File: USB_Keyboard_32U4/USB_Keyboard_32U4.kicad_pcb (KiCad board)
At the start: 2 copper layers, 36 x 14.2 mm, 14 parts, among them J1 USB_C_Receptacle_USB2.0_16P, J2 Conn_02x03_Odd_Even, U1 ATmega32U4-A, Y1 16mhz

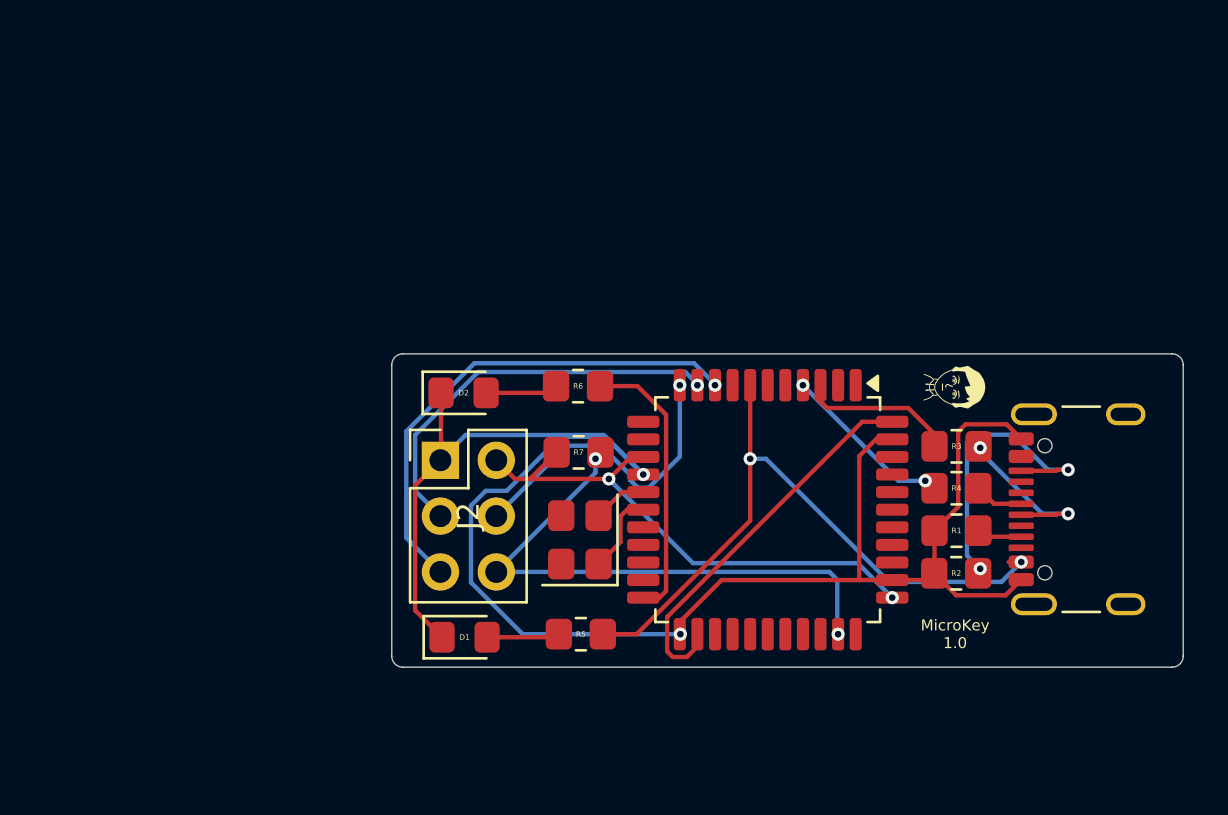
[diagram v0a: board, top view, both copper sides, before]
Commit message: Updated schematic, pcb and bom.
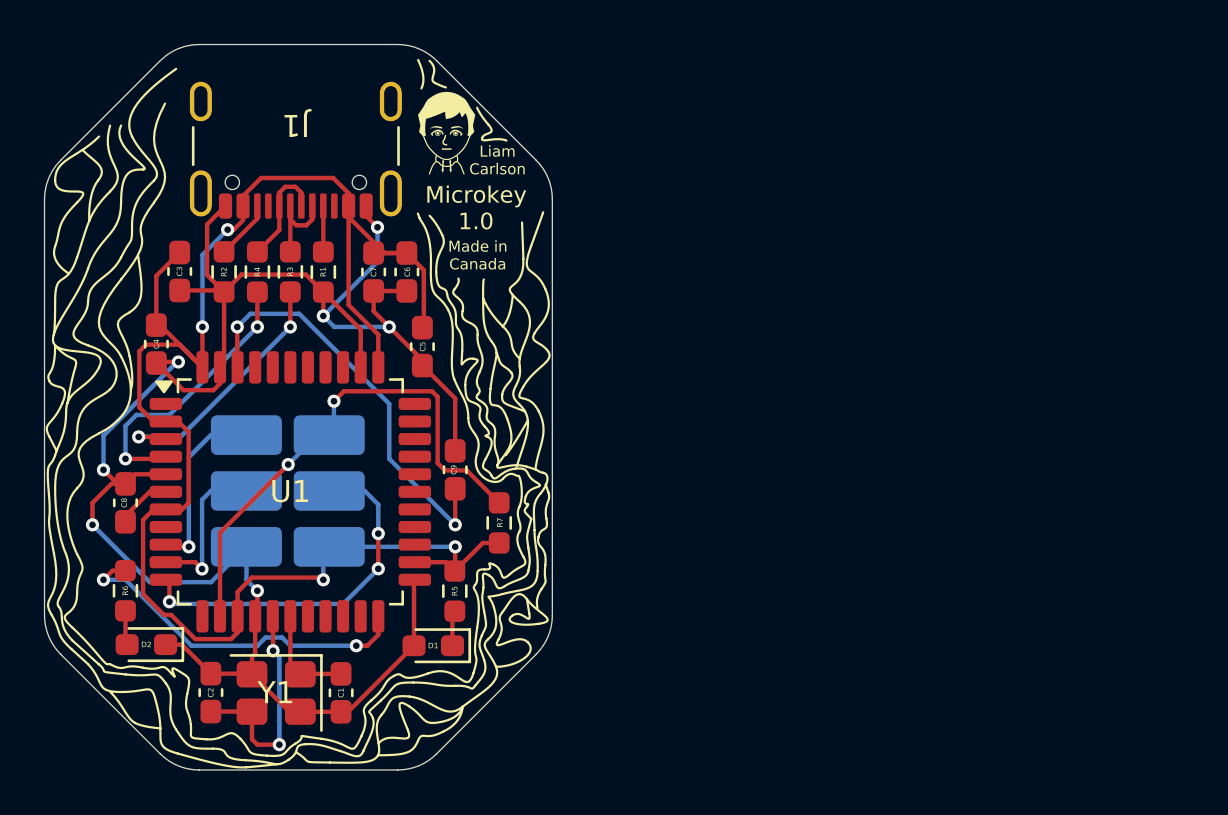
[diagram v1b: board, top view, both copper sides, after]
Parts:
- removed the G*** at (194.5, 132.9)
- added C1: 27pF, Capacitor_SMD:C_0603_1608Metric_Pad1.08x0.95mm_HandSolder, F.Cu at (166.5, 146.8)
- added C2: 27pF, Capacitor_SMD:C_0603_1608Metric_Pad1.08x0.95mm_HandSolder, F.Cu at (160.6, 146.8)
- added C3: 100nF, Capacitor_SMD:C_0603_1608Metric_Pad1.08x0.95mm_HandSolder, F.Cu at (159.2, 127.6)
- added C4: 100nF, Capacitor_SMD:C_0603_1608Metric_Pad1.08x0.95mm_HandSolder, F.Cu at (158.1, 130.9)
- added C5: 100nF, Capacitor_SMD:C_0603_1608Metric_Pad1.08x0.95mm_HandSolder, F.Cu at (170.2, 131.1)
- added C6: 100nF, Capacitor_SMD:C_0603_1608Metric_Pad1.08x0.95mm_HandSolder, F.Cu at (169.5, 127.7)
- added C7: 10uF, Capacitor_SMD:C_0603_1608Metric_Pad1.08x0.95mm_HandSolder, F.Cu at (168.0, 127.7)
- added C8: 1uF, Capacitor_SMD:C_0603_1608Metric_Pad1.08x0.95mm_HandSolder, F.Cu at (156.7, 138.2)
- added C9: 100nF, Capacitor_SMD:C_0603_1608Metric_Pad1.08x0.95mm_HandSolder, F.Cu at (171.7, 136.7)
- added G***: LOGO, Custom Footprints:MIIImage 8.25mm, F.Cu at (171.3, 121.1)
- D1, D2: footprint LED_SMD:LED_0805_2012Metric_Pad1.15x1.40mm_HandSolder -> LED_SMD:LED_0603_1608Metric_Pad1.05x0.95mm_HandSolder
- J2: footprint Connector_PinHeader_2.54mm:PinHeader_2x03_P2.54mm_Vertical -> 2x3 Pads:MicroKey_AVR_ISP_2x3_SMD; moved to B.Cu
- R1, R2, R3, R4, R5, R6: footprint Resistor_SMD:R_0805_2012Metric_Pad1.20x1.40mm_HandSolder -> Resistor_SMD:R_0603_1608Metric_Pad0.98x0.95mm_HandSolder
- R7: value 1k -> 10k; footprint Resistor_SMD:R_0805_2012Metric_Pad1.20x1.40mm_HandSolder -> Resistor_SMD:R_0603_1608Metric_Pad0.98x0.95mm_HandSolder
- Y1: value 16mhz -> 16MHz
- moved J1 40.6 mm to (164.4, 121.0), turned to 180 degrees
- moved R2 36.0 mm to (161.2, 127.7), turned to -90 degrees
- moved R4 32.8 mm to (162.7, 127.7), turned to -90 degrees
- moved R3 31.9 mm to (164.2, 127.7), turned to -90 degrees
- moved R1 31.1 mm to (165.7, 127.7), turned to -90 degrees
- moved R6 22.6 mm to (156.7, 142.2), turned to -90 degrees
- moved U1 21.7 mm to (164.2, 137.7), turned to 0 degrees
- moved D2 18.4 mm to (157.7, 144.6), turned to 180 degrees
- moved Y1 15.5 mm to (163.6, 146.8), turned to 180 degrees
- moved J2 7.08 mm to (164.1, 137.6)
- moved R5 6.06 mm to (171.7, 142.2), turned to -90 degrees
- moved R7 4.83 mm to (173.7, 139.1), turned to 90 degrees
- moved D1 1.48 mm to (170.7, 144.7), turned to 180 degrees
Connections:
- net /unconnected-(U1-PD5-Pad22) renamed Net-(U1-PD5)
- net Net-(J2-Pin_3) renamed PB2
- net Net-(J2-Pin_4) renamed PB3
- net Net-(J2-Pin_5) renamed PB1
- D1 pad 1: /Net-(J1-GND-PadA1) -> Net-(D1-K)
- D1 pad 2: Net-(D1-A) -> GND
- D2 pad 1: /Net-(J1-GND-PadA1) -> GND
- J1 pad A1: /Net-(J1-GND-PadA1) -> GND
- J1 pad A12: /Net-(J1-GND-PadA1) -> GND
- J1 pad A4: Net-(U1-VBUS) -> VCC
- J1 pad A9: Net-(U1-VBUS) -> VCC
- J1 pad B1: /Net-(J1-GND-PadA1) -> GND
- J1 pad B12: /Net-(J1-GND-PadA1) -> GND
- J1 pad B4: Net-(U1-VBUS) -> VCC
- J1 pad B6: unconnected-(J1-D+-PadB6) -> Net-(J1-D+-PadA6)
- J1 pad B7: unconnected-(J1-D--PadB7) -> Net-(J1-D--PadA7)
- J1 pad B9: Net-(U1-VBUS) -> VCC
- J1 pad SH: unconnected-(J1-SHIELD-PadSH) -> GND
- J2 pad 1: /Net-(J1-GND-PadA1) -> GND
- J2 pad 2: Net-(J2-Pin_2) -> VCC
- J2 pad 6: Net-(J2-Pin_6) -> RESET
- R1 pad 2: /Net-(J1-GND-PadA1) -> GND
- R2 pad 2: /Net-(J1-GND-PadA1) -> GND
- R3 pad 2: Net-(U1-D+) -> D-
- R4 pad 2: Net-(U1-D-) -> D+
- R5 pad 1: Net-(D1-A) -> VCC
- R5 pad 2: Net-(U1-VBUS) -> Net-(D1-K)
- R7 pad 1: Net-(J2-Pin_6) -> VCC
- R7 pad 2: Net-(J2-Pin_2) -> RESET
- U1 pad 13: unconnected-(U1-~{RESET}-Pad13) -> RESET
- U1 pad 14: Net-(J2-Pin_2) -> VCC
- U1 pad 15: /Net-(J1-GND-PadA1) -> GND
- U1 pad 2: unconnected-(U1-UVCC-Pad2) -> VCC
- U1 pad 23: /Net-(J1-GND-PadA1) -> GND
- U1 pad 24: Net-(U1-AVCC-Pad24) -> VCC
- U1 pad 3: Net-(U1-D-) -> D-
- U1 pad 32: Net-(J2-Pin_6) -> unconnected-(U1-PC7-Pad32)
- U1 pad 34: Net-(J2-Pin_2) -> VCC
- U1 pad 35: /Net-(J1-GND-PadA1) -> GND
- U1 pad 4: Net-(U1-D+) -> D+
- U1 pad 42: unconnected-(U1-AREF-Pad42) -> Net-(U1-AREF)
- U1 pad 43: /Net-(J1-GND-PadA1) -> GND
- U1 pad 44: Net-(U1-AVCC-Pad24) -> VCC
- U1 pad 5: unconnected-(U1-UGND-Pad5) -> GND
- U1 pad 6: unconnected-(U1-UCAP-Pad6) -> Net-(U1-UCAP)
- U1 pad 7: Net-(U1-VBUS) -> VCC
- Y1 pad 2: Net-(U1-XTAL2) -> GND
- Y1 pad 3: (no net) -> Net-(U1-XTAL2)
- Y1 pad 4: (no net) -> GND
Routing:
- net GND: track 0.00 -> 90.3 mm, vias 0 -> 7
- net /Net-(J1-GND-PadA1): track 81.7 -> 0.00 mm, vias 2 -> 0
- net VCC: track 0.00 -> 79.8 mm, vias 0 -> 4
- net Net-(U1-VBUS): track 30.6 -> 0.00 mm, vias 2 -> 0
- net Net-(J2-Pin_6): track 25.6 -> 0.00 mm, vias 2 -> 0
- net Net-(J2-Pin_2): track 24.3 -> 0.00 mm, vias 2 -> 0
- net RESET: track 0.00 -> 23.8 mm, vias 0 -> 2
- net Net-(U1-AREF): track 0.00 -> 19.1 mm, vias 0 -> 2
- net Net-(U1-AVCC-Pad24): track 17.7 -> 0.00 mm
- net PB1: track 22.8 -> 8.20 mm
- net D+: track 0.00 -> 12.8 mm, vias 0 -> 2
- net D-: track 0.00 -> 11.8 mm, vias 0 -> 2
- net PB2: track 18.5 -> 7.10 mm
- net Net-(J1-CC2): track 13.8 -> 2.71 mm, vias 2 -> 0
- net Net-(U1-XTAL2): track 2.48 -> 10.4 mm, vias 0 -> 2
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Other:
- board size 36 x 14.2 mm -> 23.1 x 33 mm
- board text added: "GND"
- board text added: "Liam Carlson"
- board text added: "Made in Canada"
- board text added: "Microkey 1.0"
- board text added: "PB1"
- board text added: "PB2"
- board text added: "PB3"
- board text added: "Reset"
- board text added: "VCC"

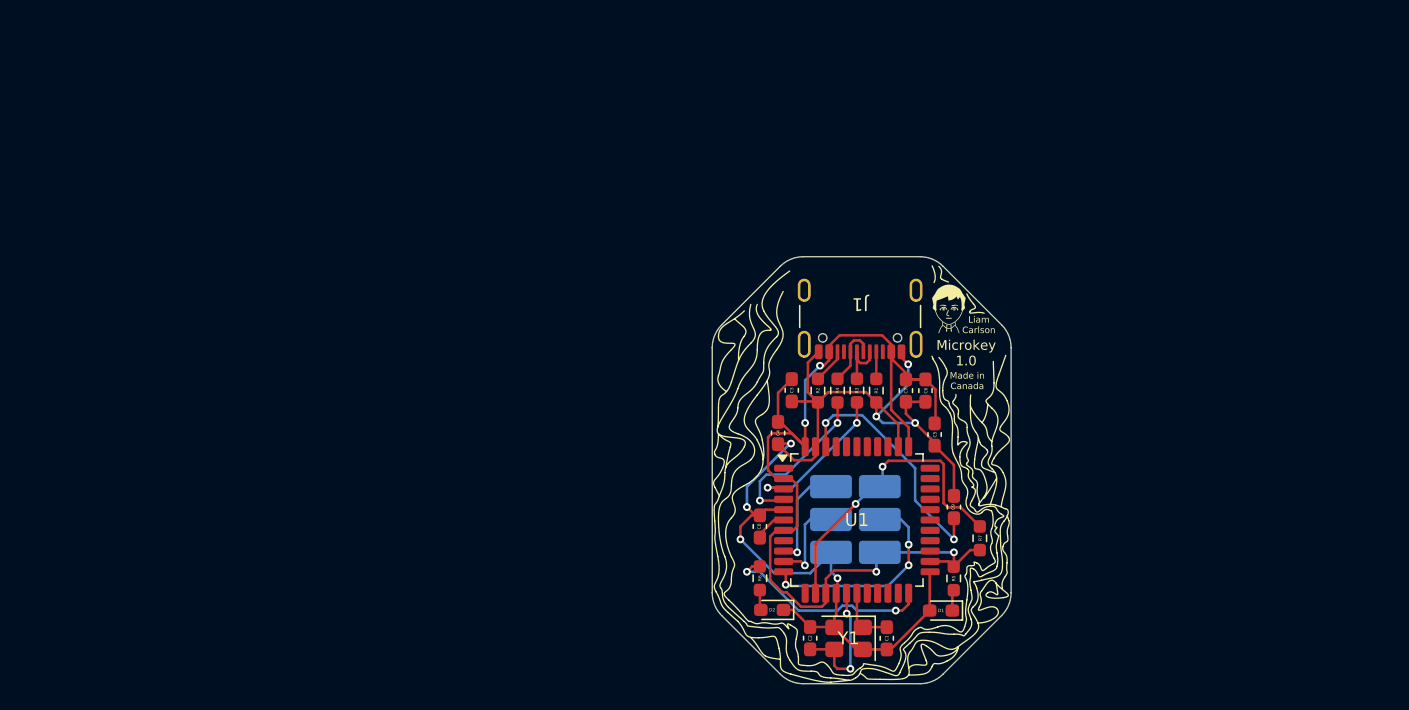
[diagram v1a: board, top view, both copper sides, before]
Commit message: Added a folder with finished files.
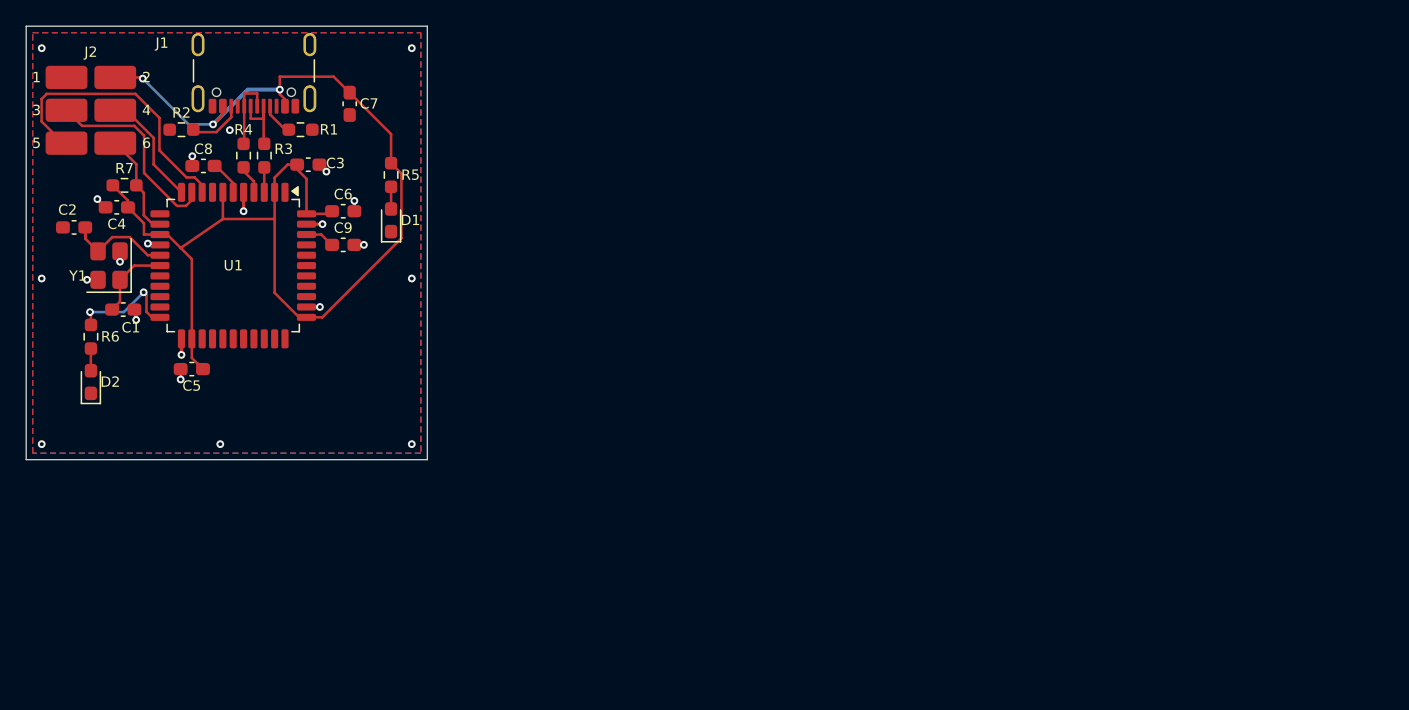
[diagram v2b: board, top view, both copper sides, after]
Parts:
- removed G***: LOGO, Custom Footprints:MIIImage 8.25mm
- J2: moved to F.Cu
- moved R7 71.5 mm to (107.6, 111.8), turned to 0 degrees
- moved J2 67.0 mm to (105.0, 106.0)
- moved C2 65.1 mm to (103.7, 115.0), turned to 0 degrees
- moved C1 64.2 mm to (107.5, 121.4), turned to 180 degrees
- moved Y1 64.0 mm to (106.4, 118.0), turned to 90 degrees
- moved C5 57.6 mm to (112.8, 126.0), turned to 180 degrees
- moved D2 55.5 mm to (105.0, 127.0), turned to 90 degrees
- moved R6 55.0 mm to (105.0, 123.5)
- moved C4 54.0 mm to (107.0, 113.5), turned to 180 degrees
- moved R5 53.5 mm to (128.2, 111.0)
- moved R2 53.2 mm to (112.0, 107.5), turned to 180 degrees
- moved D1 52.1 mm to (128.2, 114.5), turned to 90 degrees
- moved U1 52.1 mm to (116.0, 118.0), turned to -90 degrees
- moved C9 51.4 mm to (124.5, 116.4), turned to 0 degrees
- moved C8 51.2 mm to (113.7, 110.3), turned to 180 degrees
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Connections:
- D1 pad 1: Net-(D1-K) -> GND
- D1 pad 2: GND -> Net-(D1-A)
- R5 pad 2: Net-(D1-K) -> Net-(D1-A)
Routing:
- net GND: track 90.3 -> 13.1 mm, vias 7 -> 22
- net VCC: track 79.8 -> 97.6 mm, vias 4 -> 3
- net Net-(U1-AREF): track 19.1 -> 2.31 mm, vias 2 -> 0
- net RESET: track 23.8 -> 8.02 mm, vias 2 -> 0
- net PB1: track 8.20 -> 21.9 mm, vias 1 -> 0
- net D+: track 12.8 -> 2.26 mm, vias 2 -> 0
- net D-: track 11.8 -> 1.93 mm, vias 2 -> 0
- net PB2: track 7.10 -> 15.2 mm, vias 1 -> 0
- net PB3: track 16.7 -> 8.94 mm, vias 3 -> 0
- net Net-(U1-PD5): track 16.3 -> 8.62 mm
- net Net-(U1-XTAL2): track 10.4 -> 8.24 mm, vias 2 -> 0
- net Net-(U1-XTAL1): track 4.69 -> 6.53 mm
- net Net-(D1-A): track 0.00 -> 1.71 mm
- net Net-(J1-CC2): track 2.71 -> 4.35 mm
- net Net-(D1-K): track 1.62 -> 0.00 mm
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- added copper zone on B.Cu, net GND
- added copper zone on F.Cu, net GND
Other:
- board size 23.1 x 33 mm -> 31 x 33.5 mm
- board text added: "1"
- board text added: "2"
- board text added: "3"
- board text added: "4"
- board text added: "5"
- board text added: "6"
- board text removed: "GND"
- board text removed: "Liam Carlson"
- board text removed: "Made in Canada"
- board text removed: "MicroKey 1.0"
- board text removed: "Microkey 1.0"
- board text removed: "PB1"
- board text removed: "PB2"
- board text removed: "PB3"
- board text removed: "Reset"
- board text removed: "VCC"
